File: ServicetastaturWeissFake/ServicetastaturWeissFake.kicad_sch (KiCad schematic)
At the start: 65 parts, among them J1 Automat, SW1 Gewinn, SW10 Lautspr./, SW11 ↓0,10, SW12 ↑0,10, SW13 ↓Serie, SW14 ↑Serie, SW15 Zeit, SW16 ↑1,-, SW17 ↙0,10, SW18 ↙1,-, SW19 Auszahlquote, SW2 Foul, SW20 ↙5,-, SW21 Münzsp., SW22 Sp.Zähl, SW23 Lampen, SW24 Reset, SW25 Initialisieren, SW26 Münzung, SW27 Ende, SW28 ↑0,10, SW29 ↓Serie, SW3 ↙2,-, SW30 ↑Serie, SW31 ↓1,-, SW32 ↑1,-, SW4 HW-Test, SW5 Münzsp., SW6 Sp.Zähl, SW7 Dauerlauf, SW8 Reset, SW9 Initialisieren, U1 CC56-12CGKWA, U2 CC56-12CGKWA, U3 74LS48, U4 74LS145

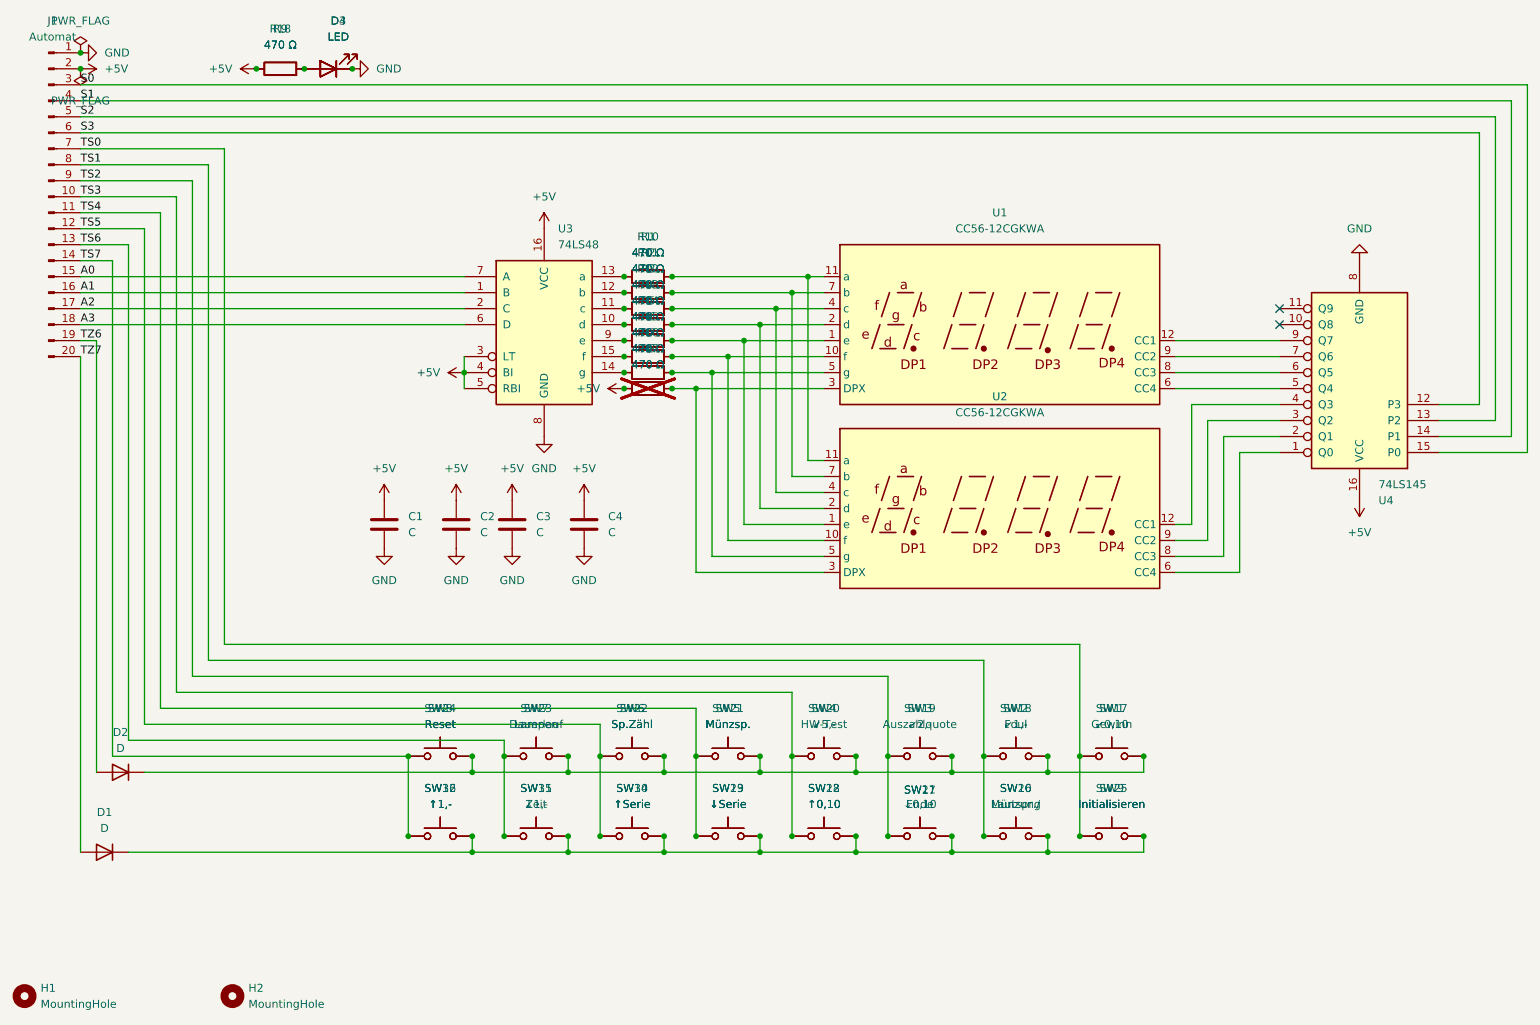
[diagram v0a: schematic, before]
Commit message: doppelIC
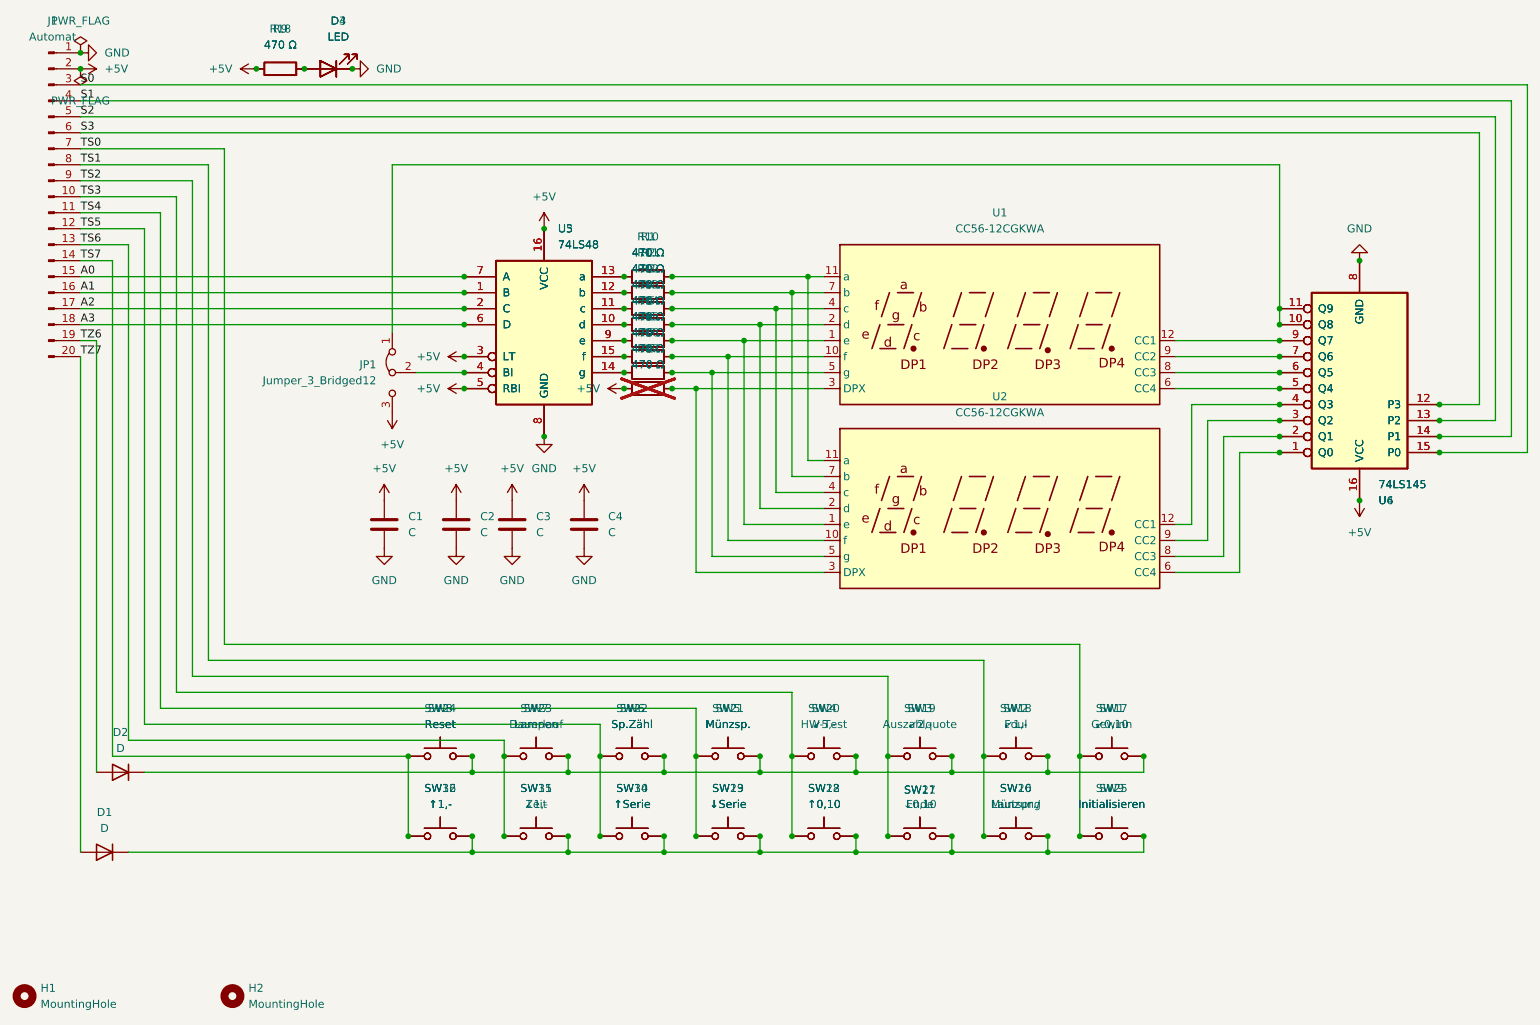
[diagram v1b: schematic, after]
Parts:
- added JP1: Jumper_3_Bridged12, Jumper:SolderJumper-3_P1.3mm_Bridged12_Pad1.0x1.5mm_NumberLabels, symbol Jumper:Jumper_3_Bridged12
- added U5: 74LS48, Package_SO:SOIC-16_4.55x10.3mm_P1.27mm, symbol 74xx:74LS48
- added U6: 74LS145, Package_SO:SOIC-16_4.55x10.3mm_P1.27mm, symbol 74xx:74LS145
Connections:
- net +5V: now also JP1.3 (B), U5.16 (VCC), U5.3 (LT), U5.5 (RBI), U6.16 (VCC); no longer U3.4 (BI)
- net A0: now also U5.7 (A)
- net A1: now also U5.1 (B)
- net A2: now also U5.2 (C)
- net A3: now also U5.6 (D)
- net GND: now also U5.8 (GND), U6.8 (GND)
- net S0: now also U6.15 (P0)
- net S1: now also U6.14 (P1)
- net S2: now also U6.13 (P2)
- net S3: now also U6.12 (P3)
- net at U1.12 (CC1), U4.9 (Q7): now also U6.9 (Q7)
- net at U1.6 (CC4), U4.5 (Q4): now also U6.5 (Q4)
- net at U1.8 (CC3), U4.6 (Q5): now also U6.6 (Q5)
- net at U1.9 (CC2), U4.7 (Q6): now also U6.7 (Q6)
- net at R15.1, R6.1, U3.15 (f): now also U5.15 (f)
- net at R13.1, R4.1, U3.10 (d): now also U5.10 (d)
- net at R11.1, R2.1, U3.12 (b): now also U5.12 (b)
- net at R12.1, R3.1, U3.11 (c): now also U5.11 (c)
- net at R16.1, R7.1, U3.14 (g): now also U5.14 (g)
- net at R1.1, R10.1, U3.13 (a): now also U5.13 (a)
- net at R14.1, R5.1, U3.9 (e): now also U5.9 (e)
- net at U2.6 (CC4), U4.1 (Q0): now also U6.1 (Q0)
- net at U4.10 (Q8): now also U4.11 (Q9), JP1.1 (A), U6.10 (Q8), U6.11 (Q9)
- net at U2.8 (CC3), U4.2 (Q1): now also U6.2 (Q1)
- net at U2.9 (CC2), U4.3 (Q2): now also U6.3 (Q2)
- net at U2.12 (CC1), U4.4 (Q3): now also U6.4 (Q3)
- new net: JP1.2 (C), U3.4 (BI), U5.4 (BI)
- no-connect marks 2 -> 0
